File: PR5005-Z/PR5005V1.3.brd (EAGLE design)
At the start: 69.8 x 69.8 mm, 29 parts, among them U1 TPA2005D1DGN

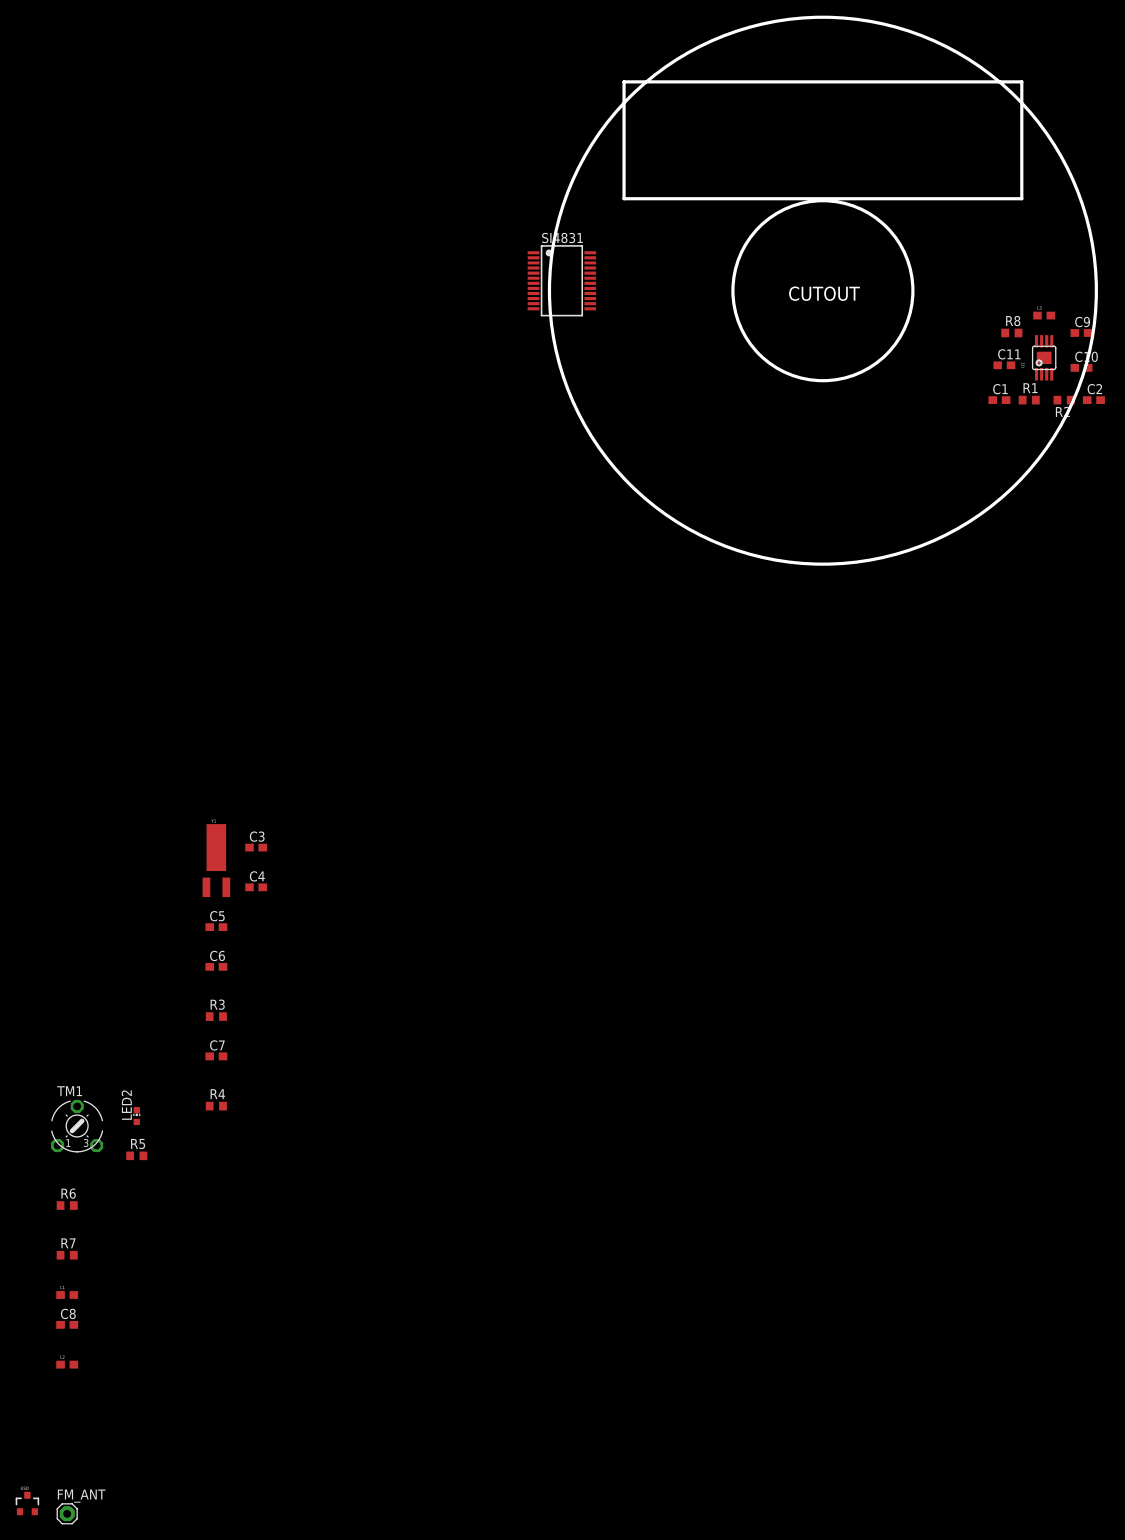
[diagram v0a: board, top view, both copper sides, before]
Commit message: PR V1.3
Updated Schematic and Layout
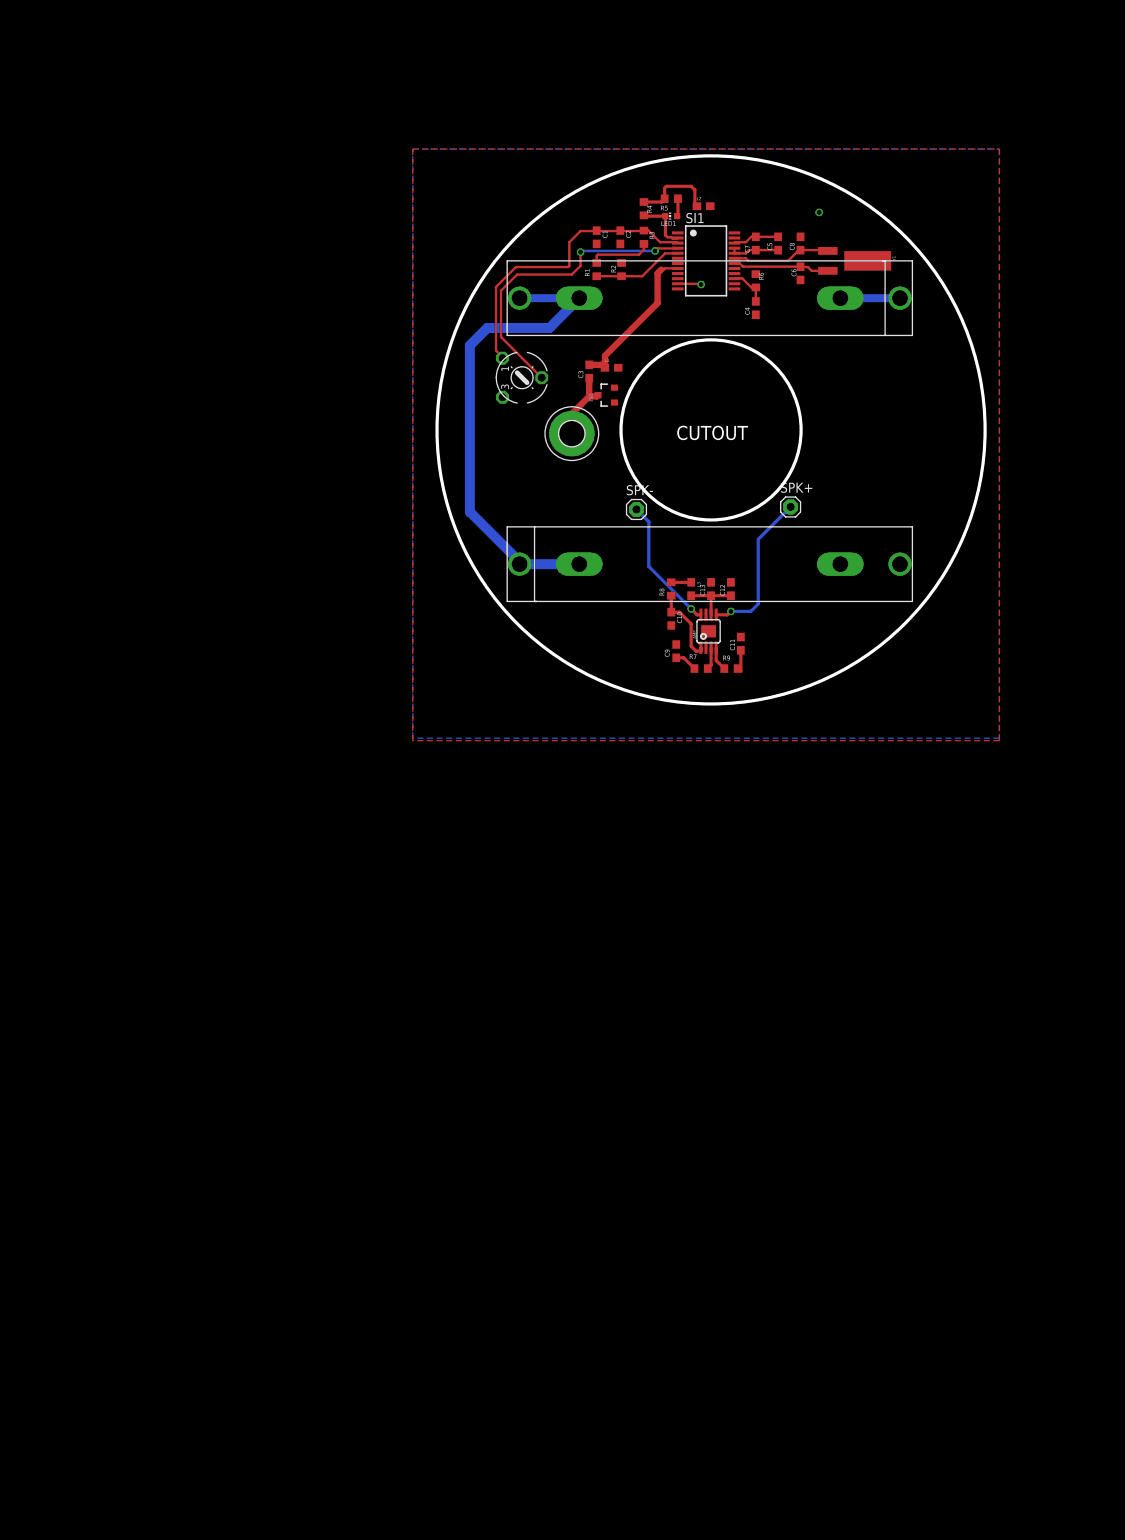
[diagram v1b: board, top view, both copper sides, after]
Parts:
- removed LED2: (no value), adafruit:CHIP-LED0603
- removed SI4831: (no value), PublicRadioICs:SI4831-SSOP-24
- removed TM1: 100K, adafruit:6MM
- removed U1: TPA2005D1DGN, SparkFun-AnalogIC:POWER-SOP8
- added AMP: TPA2005D1DGN, SparkFun-AnalogIC:POWER-SOP8
- added C12: 10uf, resistor:C0603
- added C13: 1uf, resistor:C0603
- added LED1: (no value), adafruit:CHIP-LED0603
- added R9: 59K, resistor:R0603
- added SI1: (no value), PublicRadioICs:SI4831-SSOP-24
- added SPK+, SPK-: (no value), adafruit:1X01
- added TUNE: 100K, adafruit:6MM
- added U$1, U$2: MPD-BK-92-AA-CLIP, BatteryPack:MPD-BK-92-AA-CLIP
- C1: value 1uf -> 47uF
- C11: value 10uf -> 1uf
- C2: value 1uf -> .1uF
- C3: value .1uf -> 1nF
- C4: value 4.7uf -> .1uf
- C5: value 22pF -> .1uf
- C7: value .1uf -> 4.7uf
- C8: value 1nF -> 22pF
- FM_ANT: value (none) -> MOUNT-PAD-ROUND3.2; device adafruit:1X01 -> holes:3,2-PAD
- R1: value 59K -> 412K
- R2: value 59K -> 77K
- R3: value 100K -> 1K
- R6: value 77K -> 100K
- R7: value 413K -> 59K
- moved L2 168.8 mm to (35.6, 61.6)
- moved C8 166.9 mm to (47.9, 56.8), turned to 90 degrees
- moved ESD 159.8 mm to (23.2, 37.5), turned to 90 degrees
- moved FM_ANT 152.3 mm to (18.7, 32.5)
- moved R6 147.3 mm to (42.2, 52.1), turned to 90 degrees
- moved R5 140.0 mm to (31.4, 62.5), turned to 180 degrees
- moved L1 137.3 mm to (23.8, 41.0)
- moved R4 127.0 mm to (27.9, 61.3), turned to 90 degrees
- moved C7 124.6 mm to (42.2, 56.8), turned to 90 degrees
- moved C6 115.8 mm to (47.9, 53.0), turned to 270 degrees
- moved R3 113.5 mm to (27.9, 57.6), turned to 90 degrees
- moved C5 113.0 mm to (45.1, 56.8), turned to 90 degrees
- moved Y1 111.8 mm to (51.4, 54.6), turned to 270 degrees
- moved R7 110.3 mm to (35.2, 2.54)
- moved C4 97.7 mm to (42.2, 48.6), turned to 90 degrees
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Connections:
- new net N$20: R1.2, R3.1
- new net N$21: C1.1, C2.1, R3.2, SI1.3, TUNE.A
- new net N$23: AMP.5, SPK+.1
- new net N$24: AMP.8, SPK-.1
- net GND: now also AMP.7, AMP.9, C1.2, C12.2, C13.2, C4.1, C8.2, R2.1, SI1.10, SI1.11, SI1.13, SI1.14, SI1.16, SI1.17, SI1.9, TUNE.E, U$2.-, U$2.-1; no longer C5.2, C7.1, C9.2, R6.1, SI4831.10, SI4831.11, SI4831.13, SI4831.14, SI4831.16, SI4831.17, SI4831.9, TM1.E, U1.7, U1.9
- net N$1: now also AMP.3, R7.2; no longer R1.2, U1.3
- net N$10: now also SI1.18, Y1.X2; no longer SI4831.18, Y1.X1
- net N$11: now also LED1.A; no longer LED2.A
- net N$12: now also SI1.4, TUNE.S; no longer SI4831.4, TM1.S
- net N$13: now also R1.1, R2.2, SI1.5; no longer R6.2, R7.2, SI4831.5
- net N$14: now also U$1.-, U$1.-1, U$2.+, U$2.+1; no longer R7.1, SI4831.3, TM1.A
- net N$15: now also C3.2, SI1.8; no longer C8.2, SI4831.8
- net N$16: now also C5.1, C7.1, SI1.20, SI1.21; no longer C3.1, C4.1, SI4831.20, SI4831.21
- net N$17: now also AMP.6, C12.1, C13.1; no longer C10.1, C9.1, U1.6
- net N$18: now also AMP.1, C10.1; no longer C11.1, U1.1
- net N$19: now also C3.1, FM_ANT.B3,2; no longer C8.1, FM_ANT.1
- net N$2: now also AMP.4, R9.2; no longer R2.2, U1.4
- net N$3: now also C11.1, R9.1; no longer C2.1, R2.1
- net N$4: now also C9.2, R7.1; no longer C1.2, R1.1
- net N$5: now also C9.1, SI1.24; no longer C1.1, SI4831.24
- net N$6: now also C5.2, C7.2, SI1.22; no longer C3.2, C4.2, SI4831.22
- net N$7: now also C8.1, SI1.19, Y1.X1; no longer C5.1, SI4831.19, Y1.X2
- net N$8: now also C4.2, R6.1, SI1.15; no longer C7.2, R3.1, SI4831.15
- net N$9: now also LED1.C, SI1.2; no longer LED2.C, SI4831.2
- net VCC: now also R6.2, U$1.+, U$1.+1; no longer R3.2
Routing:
- net N$14: track 0.00 -> 62.4 mm
- net N$12: track 0.00 -> 39.1 mm, vias 0 -> 2
- net N$21: track 0.00 -> 38.1 mm
- net VCC: track 0.00 -> 20.7 mm
- net N$23: track 0.00 -> 20.0 mm, vias 0 -> 1
- net N$15: track 0.00 -> 19.9 mm
- net N$24: track 0.00 -> 17.2 mm, vias 0 -> 1
- net N$7: track 0.00 -> 12.7 mm
- net N$10: track 0.00 -> 12.3 mm
- net N$13: track 0.00 -> 11.6 mm
- net N$18: track 0.00 -> 10.1 mm
- net N$19: track 0.00 -> 9.20 mm
- net N$20: track 0.00 -> 8.00 mm
- net N$17: track 0.00 -> 7.53 mm
- net N$9: track 0.00 -> 6.99 mm
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- added copper zone on layer 1, net GND
- added copper zone on layer 16, net N$22
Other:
- board size 69.8 x 69.8 mm -> 70 x 70 mm
